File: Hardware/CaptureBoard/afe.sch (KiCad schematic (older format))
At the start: 41 parts, among them U1 ADA4800, U2 ADA4800, U800 AD9990, Y800 30MHz

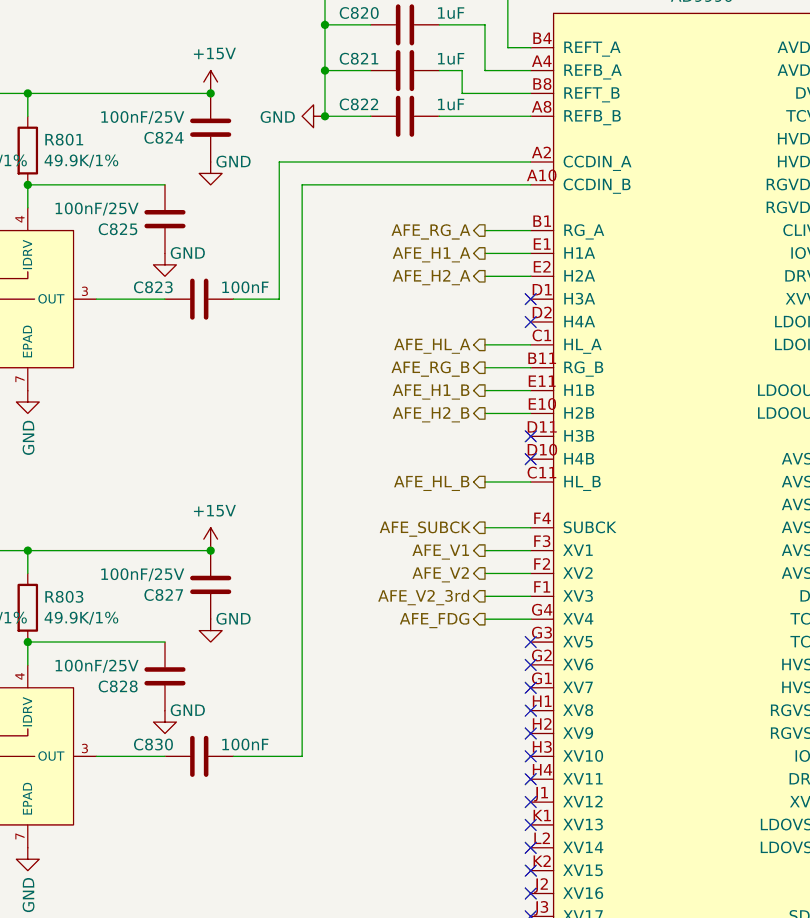
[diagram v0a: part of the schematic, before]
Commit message: pcb: working on layout
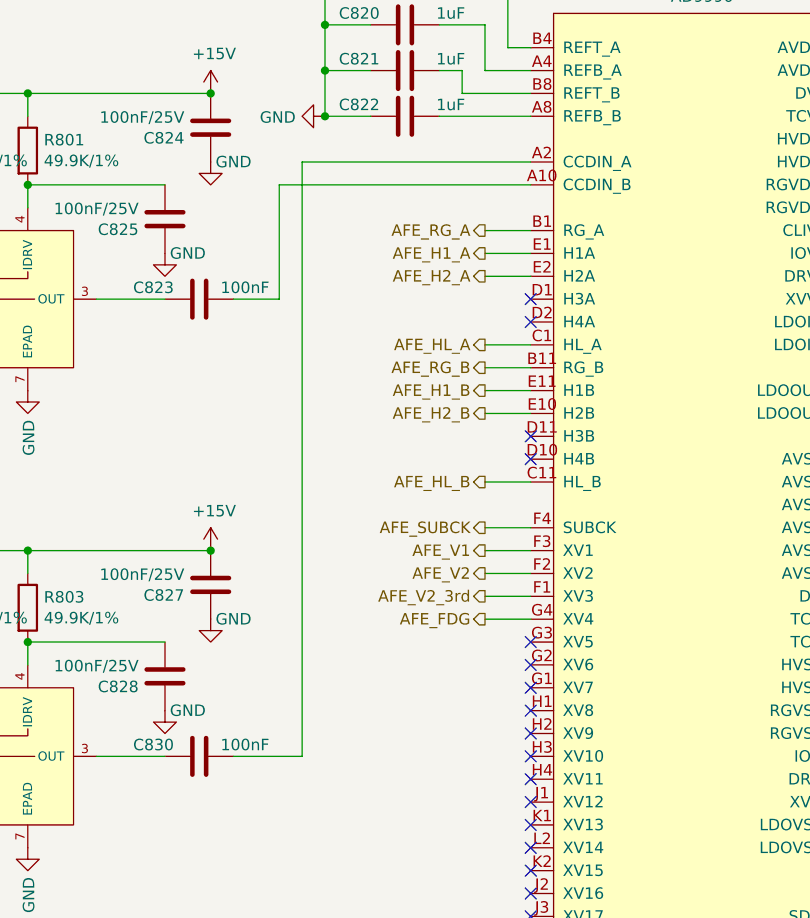
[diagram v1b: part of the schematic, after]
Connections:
- net at U800.A10 (CCDIN_B): now also C823.1; no longer C830.1
- net at U800.A2 (CCDIN_A): now also C830.1; no longer C823.1
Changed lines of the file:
@@
 	3600 2200 3800 2200
 Wire Wire Line
-	3800 2200 3800 1600
+	3800 2200 3800 1700
 Wire Wire Line
 	3600 4200 3900 4200
-Wire Wire Line
-	3900 4200 3900 1700
 $Comp
 L power:GND #PWR0222
@@
 	6500 2900 6400 2900
 Wire Wire Line
-	3800 1600 4900 1600
-Wire Wire Line
 	6500 2700 6400 2700
-Wire Wire Line
-	3900 1700 4900 1700
 Wire Wire Line
 	6400 2600 6500 2600
@@
 	6500 6900 6400 6900
 Wire Wire Line
+	4900 1700 3800 1700
+Wire Wire Line
+	4900 1600 3900 1600
+Wire Wire Line
+	3900 1600 3900 4200
+Wire Wire Line
 	6400 5400 7000 5400

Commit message: pcb: wip
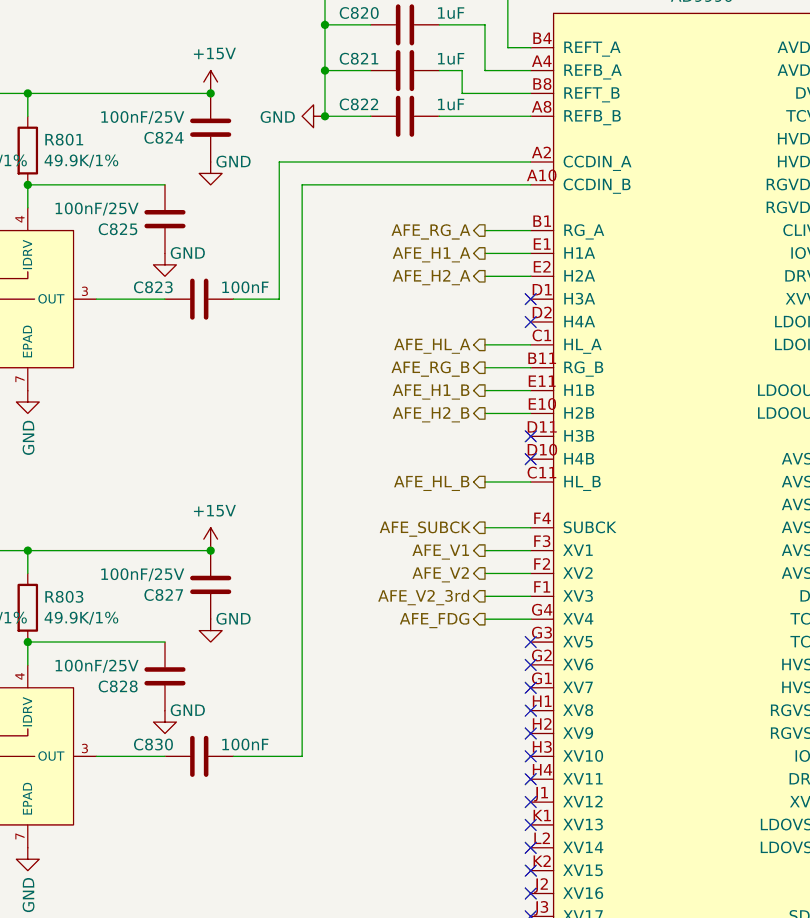
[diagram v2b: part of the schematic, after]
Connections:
- net at U800.A10 (CCDIN_B): now also C830.1; no longer C823.1
- net at U800.A2 (CCDIN_A): now also C823.1; no longer C830.1
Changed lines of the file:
@@
 	3600 2200 3800 2200
-Wire Wire Line
-	3800 2200 3800 1700
 Wire Wire Line
 	3600 4200 3900 4200
@@
 	6500 6900 6400 6900
 Wire Wire Line
-	4900 1700 3800 1700
-Wire Wire Line
-	4900 1600 3900 1600
-Wire Wire Line
-	3900 1600 3900 4200
+	3800 1600 4900 1600
+Wire Wire Line
+	3800 1600 3800 2200
+Wire Wire Line
+	4900 1700 3900 1700
+Wire Wire Line
+	3900 1700 3900 4200
 Wire Wire Line
 	6400 5400 7000 5400
